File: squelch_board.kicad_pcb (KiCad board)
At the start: 2 copper layers, 50 x 50 mm, 92 parts, among them P1 PWR, P2 DISC., P3 OUT, P4 CONN_02X04, P5 CONN-10033526-N3212LF, P6 CONN_01X05, P7 LPF, P8 HPF, P9 DISC., U1 STM32F070F6P, U2 Ricom R-786.5-0.5, U3 AP2202, U4 MCP6002, U5 MCP6002, U6 CP2105

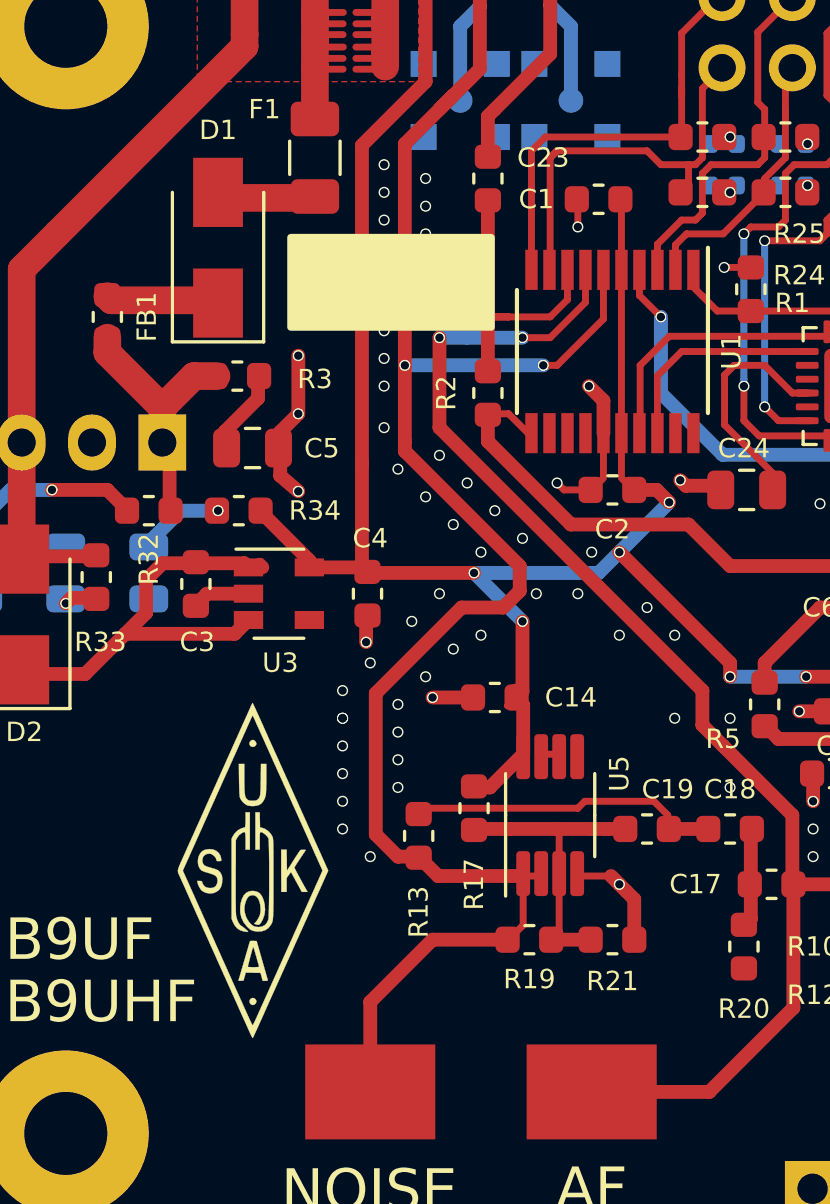
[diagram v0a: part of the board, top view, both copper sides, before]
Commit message: Changing silk screen block diagram: brin pictogram
Brain pictogrm is licensed under a CC-BY license, jessie_vp is
attributed for the original work. Source:
https://thenounproject.com/term/brain/35201/
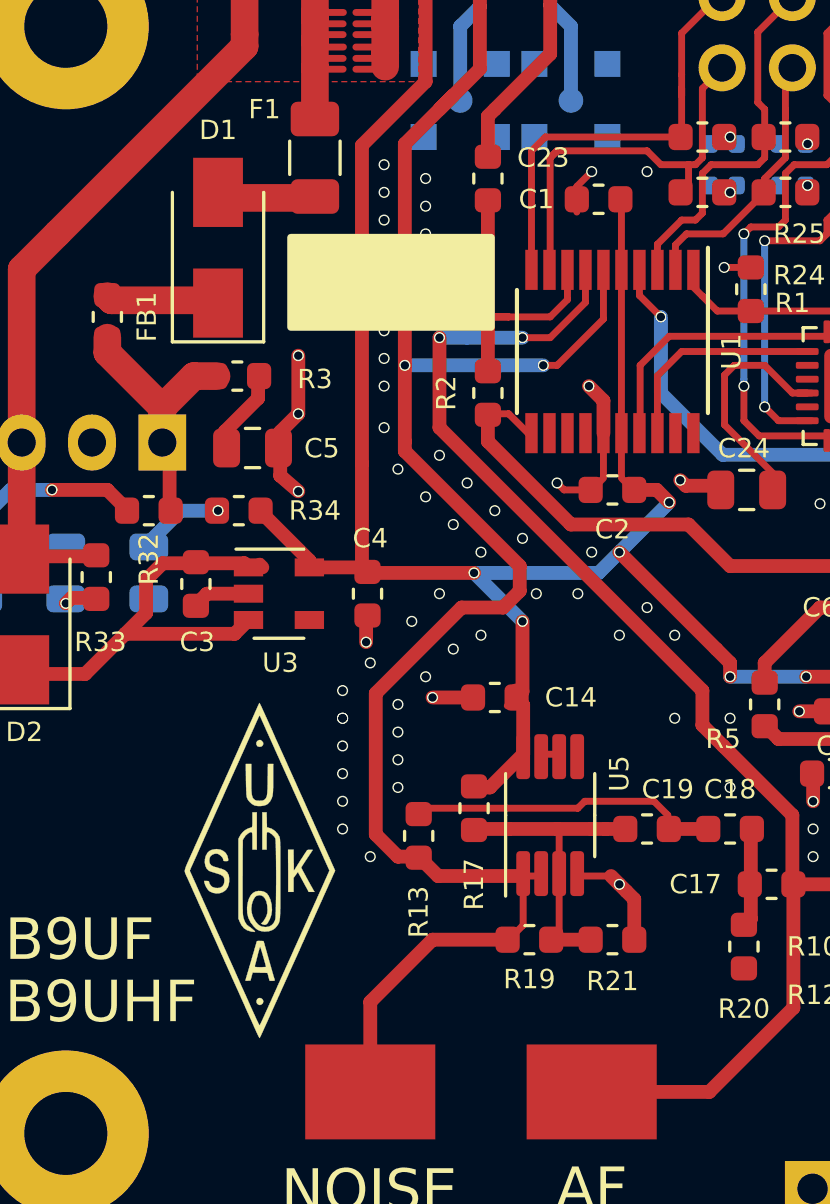
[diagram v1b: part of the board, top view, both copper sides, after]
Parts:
- added G***: LOGO, local:brain, B.Cu at (137.0, 71.8)
- moved G*** 0.25 mm to (127.0, 90.5)
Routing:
- net GND: track 45.9 -> 46.6 mm, vias 87 -> 88
